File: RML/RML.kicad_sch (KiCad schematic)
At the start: 23 parts, among them Q1 NMOS, U1 74AHC1G02, U102 641964-1, U103 641964-1, U104 LM555xM, U2 LM7805_TO220, U3 SFH617A-1

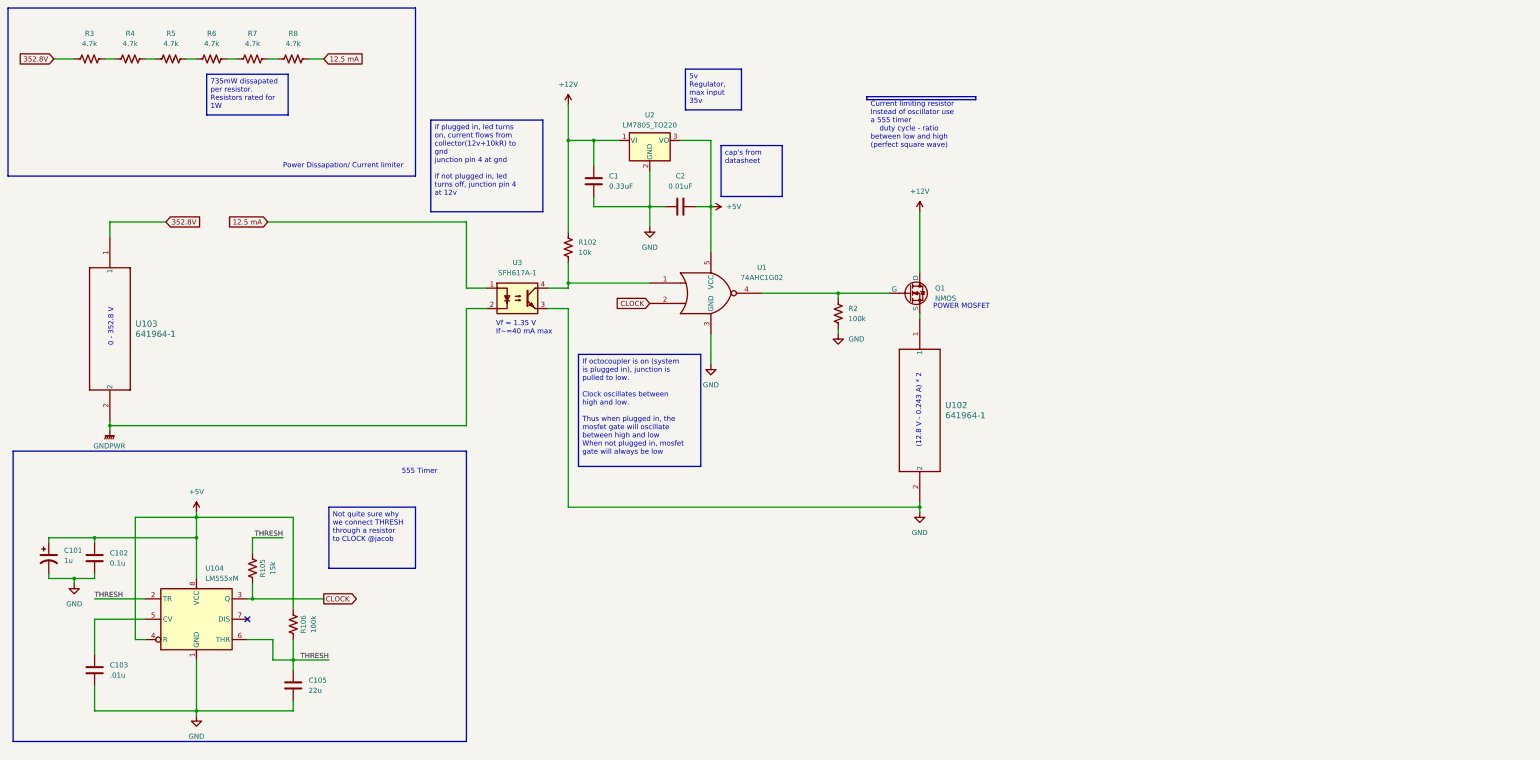
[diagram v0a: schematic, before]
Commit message: Changes to RML and TSSI
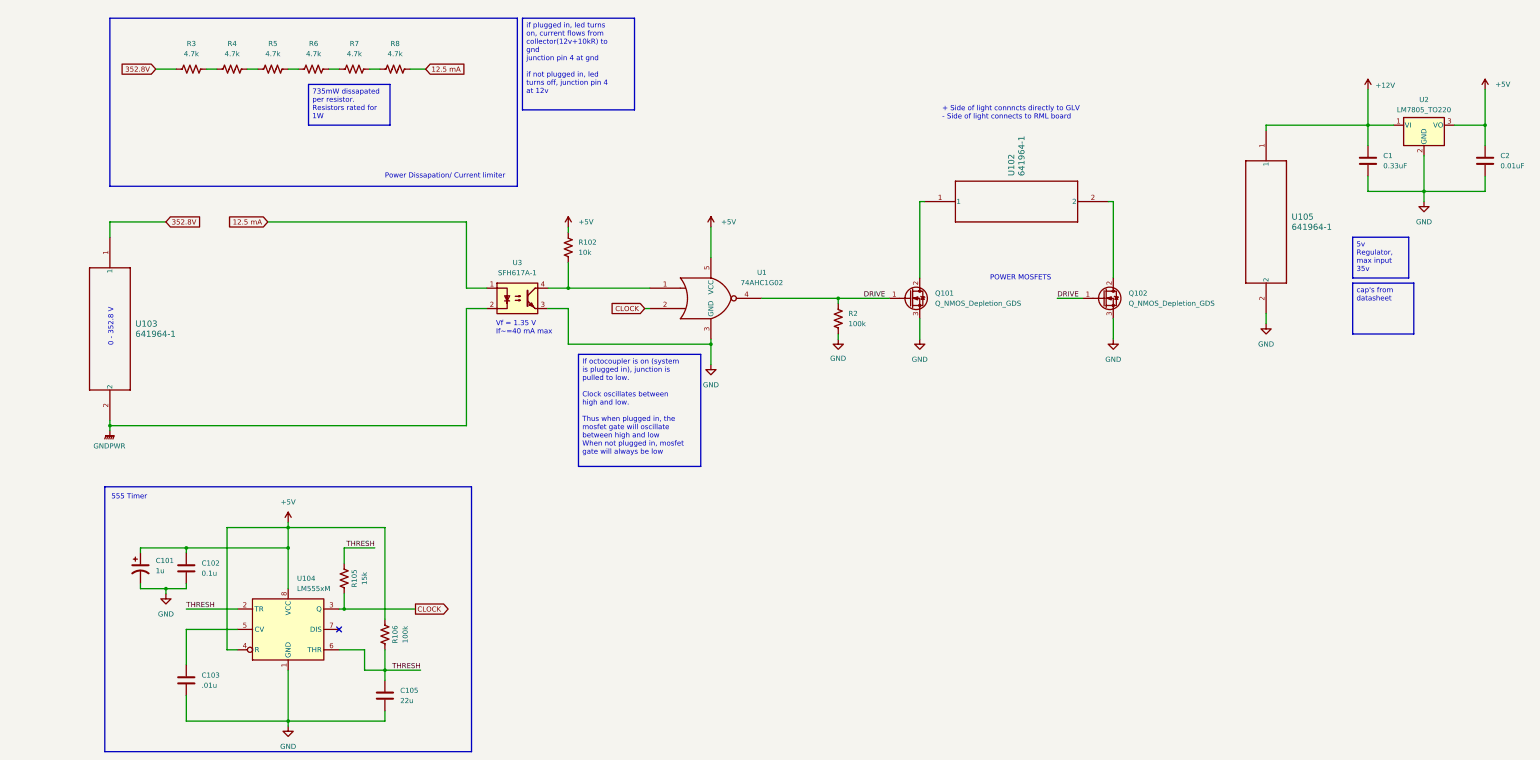
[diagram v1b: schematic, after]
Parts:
- removed Q1: NMOS, Package_TO_SOT_THT:TO-220-3_Vertical, symbol Simulation_SPICE:NMOS
- added Q101, Q102: Q_NMOS_Depletion_GDS, Package_TO_SOT_THT:TO-220-3_Vertical, symbol Transistor_FET_Other:Q_NMOS_Depletion_GDS
- added U105: 641964-1, 641964-1_TYC, symbol CONNECTOR:641964-1
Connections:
- net +12V: now also U105.1; no longer R102.1
- net +5V: now also R102.1
- net GND: now also Q101.3 (S), Q102.3 (S), U105.2; no longer U102.2
- net DRIVE: now reaches R2.2, U1.4
- net DRIVE: now also Q101.1 (G), Q102.1 (G)
- net at U102.1: now also Q101.2 (D)
- new net: Q102.2 (D), U102.2
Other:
- note added: "+ Side of light connncts directly to GLV - Side of light connects to RML board"
- note added: "POWER MOSFETS"
- note removed: "(12.8 V - 0.243 A) * 2"
- note removed: "POWER MOSFET"
- moved on the sheet: C1, C101, C102, C103, C105, C2, R105, R106, R2, R3, R4, R5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
